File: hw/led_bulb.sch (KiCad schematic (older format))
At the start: 93 parts, among them P1 USB_OTG, P10 CONN_01X04, P11 CONN_01X04, P12 CONN_01X04, P13 CONN_01X04, P14 CONN_01X04, P15 CONN_01X04, P16 CONN_01X04, P17 CONN_01X04, P2 CONN_01X04, P3 CONN_01X04, P4 CONN_01X04, P5 CONN_01X04, P6 CONN_01X04, P7 CONN_01X04, P8 CONN_01X04, P9 CONN_01X04, SW1 SW_RST, SW2 SW_FLASH, U1 CP2102, U3 ESP-12E, U4 AP1117D33

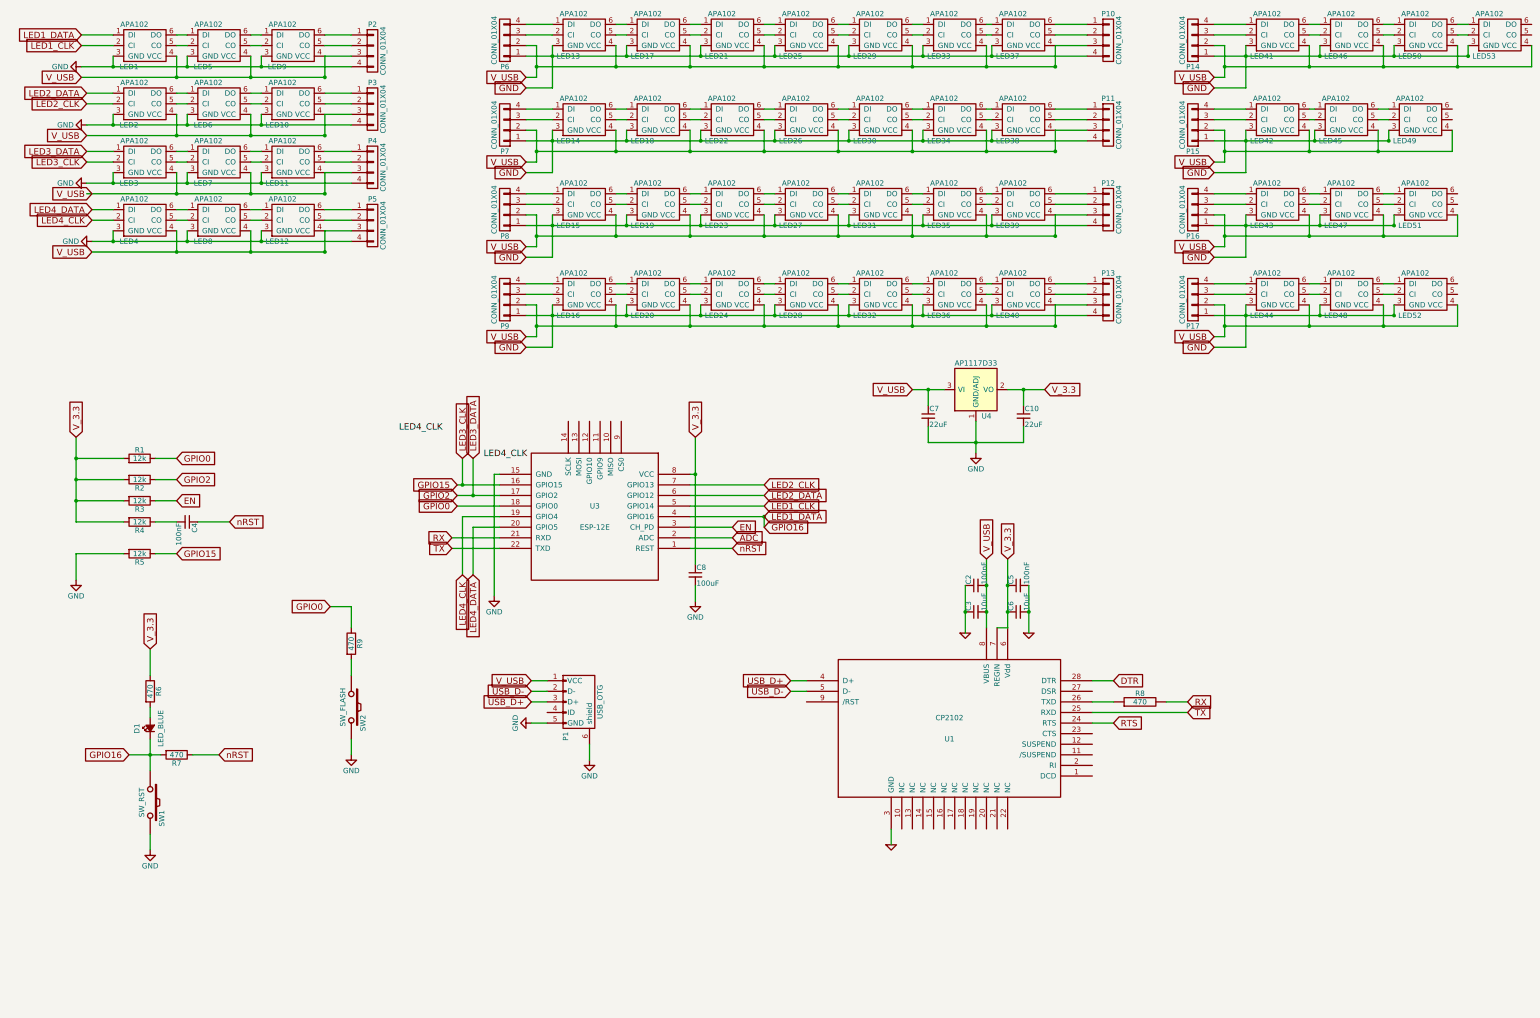
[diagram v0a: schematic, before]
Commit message: Added first version of v4 hardware.
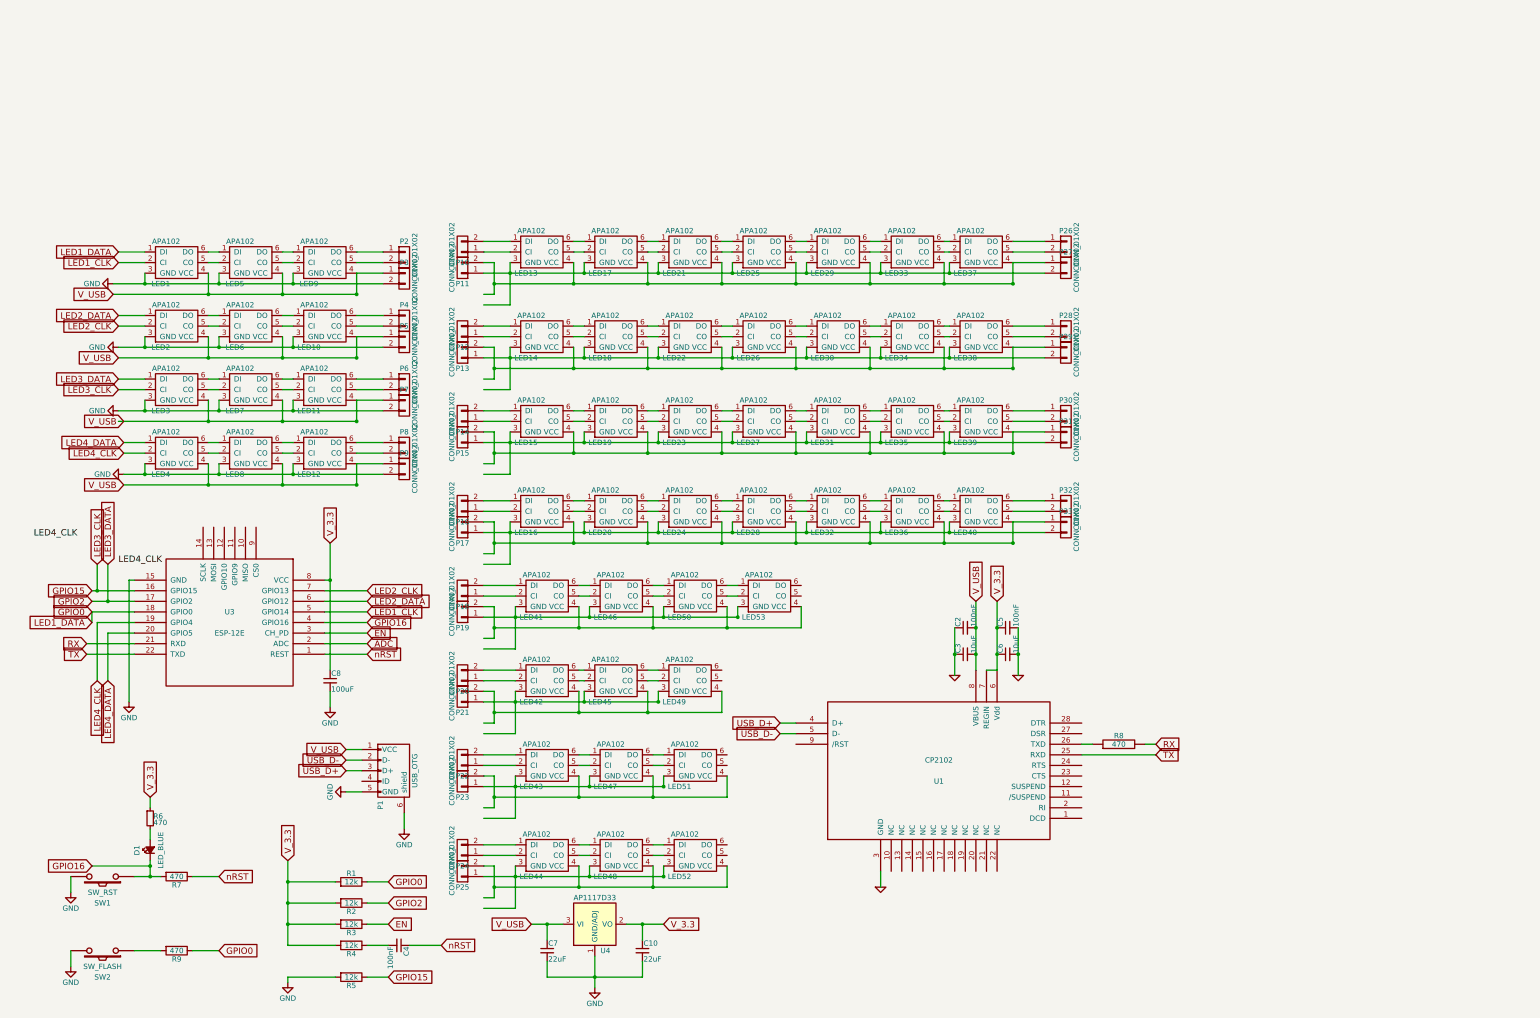
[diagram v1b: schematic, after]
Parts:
- removed P10, P11, P12, P13, P14, P15, P16, P17, P2, P3, P4, P5, P6, P7, P8, P9: CONN_01X04, Connectors:CONN_2.54mm_1x4, symbol CONN_01X04
- removed R6: 470, Resistors_SMD:R_0603, symbol R-RESCUE-led_matrix_apa102
- added P10, P11, P12, P13, P14, P15, P16, P17, P18, P19, P2, P20, P21, P22, P23, P24, P25, P26, P27, P28, P29, P3, P30, P31, P32, P33, P4, P5, P6, P7, P8, P9: CONN_01X02, footprints:CONN_2.54mm_1x2_no-outline, symbol CONN_01X02
- added R6: 470, Resistors_SMD:R_0603, symbol R_Small
- D1: footprint LEDs:LED-0603 -> Capacitors_SMD:C_0603
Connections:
- net labels removed: DTR, RTS
- wire segments 365 -> 363
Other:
- moved on the sheet: C10, C2, C3, C4, C5, C6, C7, C8, LED1, LED10, LED11, LED12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
